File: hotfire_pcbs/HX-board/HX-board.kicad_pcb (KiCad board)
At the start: 2 copper layers, 101.6 x 88.5 mm, 55 parts, among them J1 Testpoints, J2 PCIE-LP-01-01-F-DV-A-TR, J3 DB15_Female, J4 Testpoints, J5 DB15_Female, J6 Testpoints, U1 HX711_Breakout, U2 HX711_Breakout, U3 HX711_Breakout, U4 HX711_Breakout, U5 HX711_Breakout

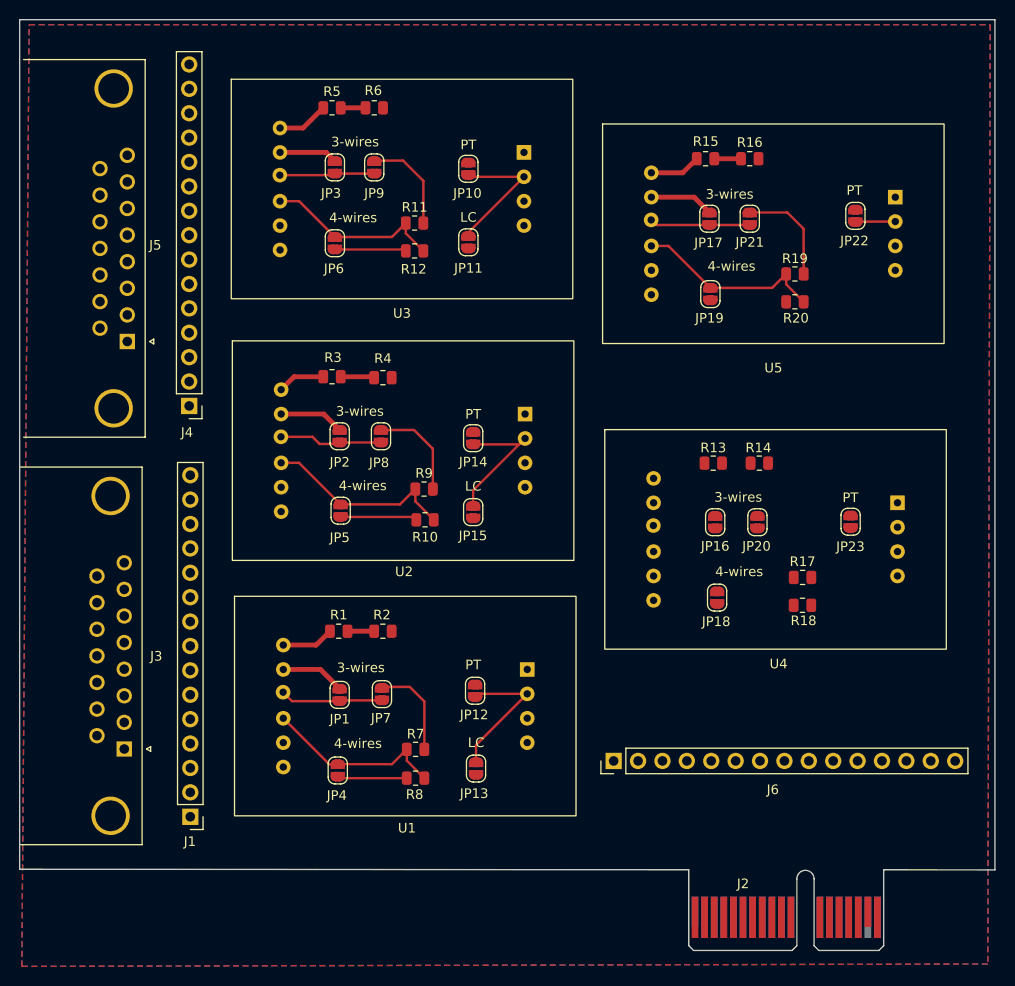
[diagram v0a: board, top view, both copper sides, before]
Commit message: Finished wiring HX. Need review + silkscreen.
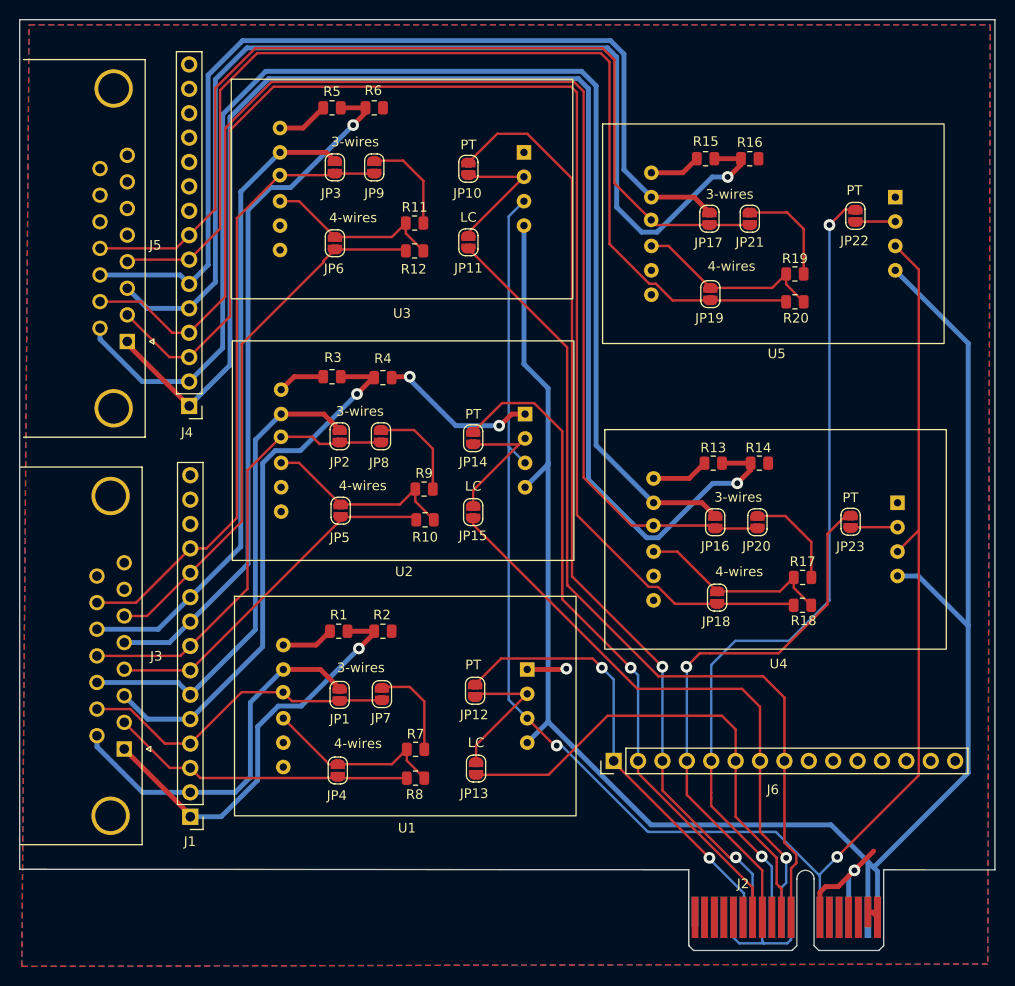
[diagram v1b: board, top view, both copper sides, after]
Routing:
- net +5V: track 0.00 -> 189.7 mm
- net /HX_CLK: track 0.00 -> 173.4 mm, vias 0 -> 2
- net /PT4_E+: track 0.00 -> 147.3 mm, vias 0 -> 1
- net /PT4_A+: track 0.00 -> 142.4 mm
- net /PT4_E-: track 0.00 -> 135.8 mm
- net /PT4_A-: track 0.00 -> 133.7 mm
- net /PT5_E+: track 2.77 -> 111.8 mm, vias 0 -> 1
- net /PT5_A+: track 0.00 -> 107.9 mm
- net /PCIe_3: track 0.00 -> 99.1 mm, vias 0 -> 2
- net /PT5_E-: track 6.71 -> 100.4 mm
- net /PCIe_8: track 0.00 -> 90.4 mm
- net /PT5_A-: track 10.5 -> 98.8 mm
- net /PCIe_5: track 0.00 -> 86.4 mm, vias 0 -> 2
- net /PCIe_2: track 0.00 -> 70.6 mm, vias 0 -> 1
- net /PT3_E+: track 2.57 -> 72.6 mm, vias 0 -> 1
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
